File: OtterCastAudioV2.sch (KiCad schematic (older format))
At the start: 23 parts, among them J1 UART, J2 SD, U1 AllWinner-S3(FBGA-234), U2 AT24CS16-MAHM

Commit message: no drc error
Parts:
- R1, R10, R11, R12, R13, R2, R3, R4, R5, R6, R7, R8, R9: footprint otter:C_0402 -> otter:R_0402
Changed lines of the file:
@@
 F 0 "R7" V 11400 7750 50  0000 C CNN
 F 1 "47k" V 11400 8100 50  0000 C CNN
-F 2 "otter:C_0402" H 11450 7900 50  0001 C CNN
+F 2 "otter:R_0402" H 11450 7900 50  0001 C CNN
 F 3 "~" H 11450 7900 50  0001 C CNN
 	1    11450 7900
@@
 F 0 "R8" V 11400 7850 50  0000 C CNN
 F 1 "47k" V 11400 8200 50  0000 C CNN
-F 2 "otter:C_0402" H 11450 8000 50  0001 C CNN
+F 2 "otter:R_0402" H 11450 8000 50  0001 C CNN
 F 3 "~" H 11450 8000 50  0001 C CNN
 	1    11450 8000
@@
 F 0 "R9" V 11400 7950 50  0000 C CNN
 F 1 "47k" V 11400 8300 50  0000 C CNN
-F 2 "otter:C_0402" H 11450 8100 50  0001 C CNN
+F 2 "otter:R_0402" H 11450 8100 50  0001 C CNN
 F 3 "~" H 11450 8100 50  0001 C CNN
 	1    11450 8100
@@
 F 0 "R10" V 11400 8150 50  0000 C CNN
 F 1 "47k" V 11400 8500 50  0000 C CNN
-F 2 "otter:C_0402" H 11450 8300 50  0001 C CNN
+F 2 "otter:R_0402" H 11450 8300 50  0001 C CNN
 F 3 "~" H 11450 8300 50  0001 C CNN
 	1    11450 8300
@@
 F 0 "R11" V 11400 8350 50  0000 C CNN
 F 1 "47k" V 11400 8700 50  0000 C CNN
-F 2 "otter:C_0402" H 11450 8500 50  0001 C CNN
+F 2 "otter:R_0402" H 11450 8500 50  0001 C CNN
 F 3 "~" H 11450 8500 50  0001 C CNN
 	1    11450 8500
@@
 F 0 "R12" V 11400 8450 50  0000 C CNN
 F 1 "47k" V 11400 8800 50  0000 C CNN
-F 2 "otter:C_0402" H 11450 8600 50  0001 C CNN
+F 2 "otter:R_0402" H 11450 8600 50  0001 C CNN
 F 3 "~" H 11450 8600 50  0001 C CNN
 	1    11450 8600
@@
 F 0 "R13" V 11400 8550 50  0000 C CNN
 F 1 "47k" V 11400 8900 50  0000 C CNN
-F 2 "otter:C_0402" H 11450 8700 50  0001 C CNN
+F 2 "otter:R_0402" H 11450 8700 50  0001 C CNN
 F 3 "~" H 11450 8700 50  0001 C CNN
 	1    11450 8700
@@
 F 0 "R3" H 8041 10346 50  0000 R CNN
 F 1 "5k1" H 8041 10255 50  0000 R CNN
-F 2 "otter:C_0402" H 8100 10300 50  0001 C CNN
+F 2 "otter:R_0402" H 8100 10300 50  0001 C CNN
 F 3 "~" H 8100 10300 50  0001 C CNN
 	1    8100 10300
@@
 F 0 "R2" V 3950 6450 50  0000 C CNN
 F 1 "DNP" V 4000 6600 50  0000 C CNN
-F 2 "otter:C_0402" H 4000 6600 50  0001 C CNN
+F 2 "otter:R_0402" H 4000 6600 50  0001 C CNN
 F 3 "~" H 4000 6600 50  0001 C CNN
 	1    4000 6600
@@
 F 0 "R4" H 8391 10346 50  0000 R CNN
 F 1 "5k1" H 8391 10255 50  0000 R CNN
-F 2 "otter:C_0402" H 8450 10300 50  0001 C CNN
+F 2 "otter:R_0402" H 8450 10300 50  0001 C CNN
 F 3 "~" H 8450 10300 50  0001 C CNN
 	1    8450 10300
@@
 F 0 "R1" V 3646 2600 50  0000 C CNN
 F 1 "5k1" V 3555 2600 50  0000 C CNN
-F 2 "otter:C_0402" H 3450 2600 50  0001 C CNN
+F 2 "otter:R_0402" H 3450 2600 50  0001 C CNN
 F 3 "~" H 3450 2600 50  0001 C CNN
 	1    3450 2600
@@
 F 0 "R5" H 10609 10246 50  0000 L CNN
 F 1 "2.2k" H 10609 10155 50  0000 L CNN
-F 2 "otter:C_0402" H 10550 10200 50  0001 C CNN
+F 2 "otter:R_0402" H 10550 10200 50  0001 C CNN
 F 3 "~" H 10550 10200 50  0001 C CNN
 	1    10550 10200
@@
 F 0 "R6" H 10859 10246 50  0000 L CNN
 F 1 "2.2k" H 10859 10155 50  0000 L CNN
-F 2 "otter:C_0402" H 10800 10200 50  0001 C CNN
+F 2 "otter:R_0402" H 10800 10200 50  0001 C CNN
 F 3 "~" H 10800 10200 50  0001 C CNN
 	1    10800 10200

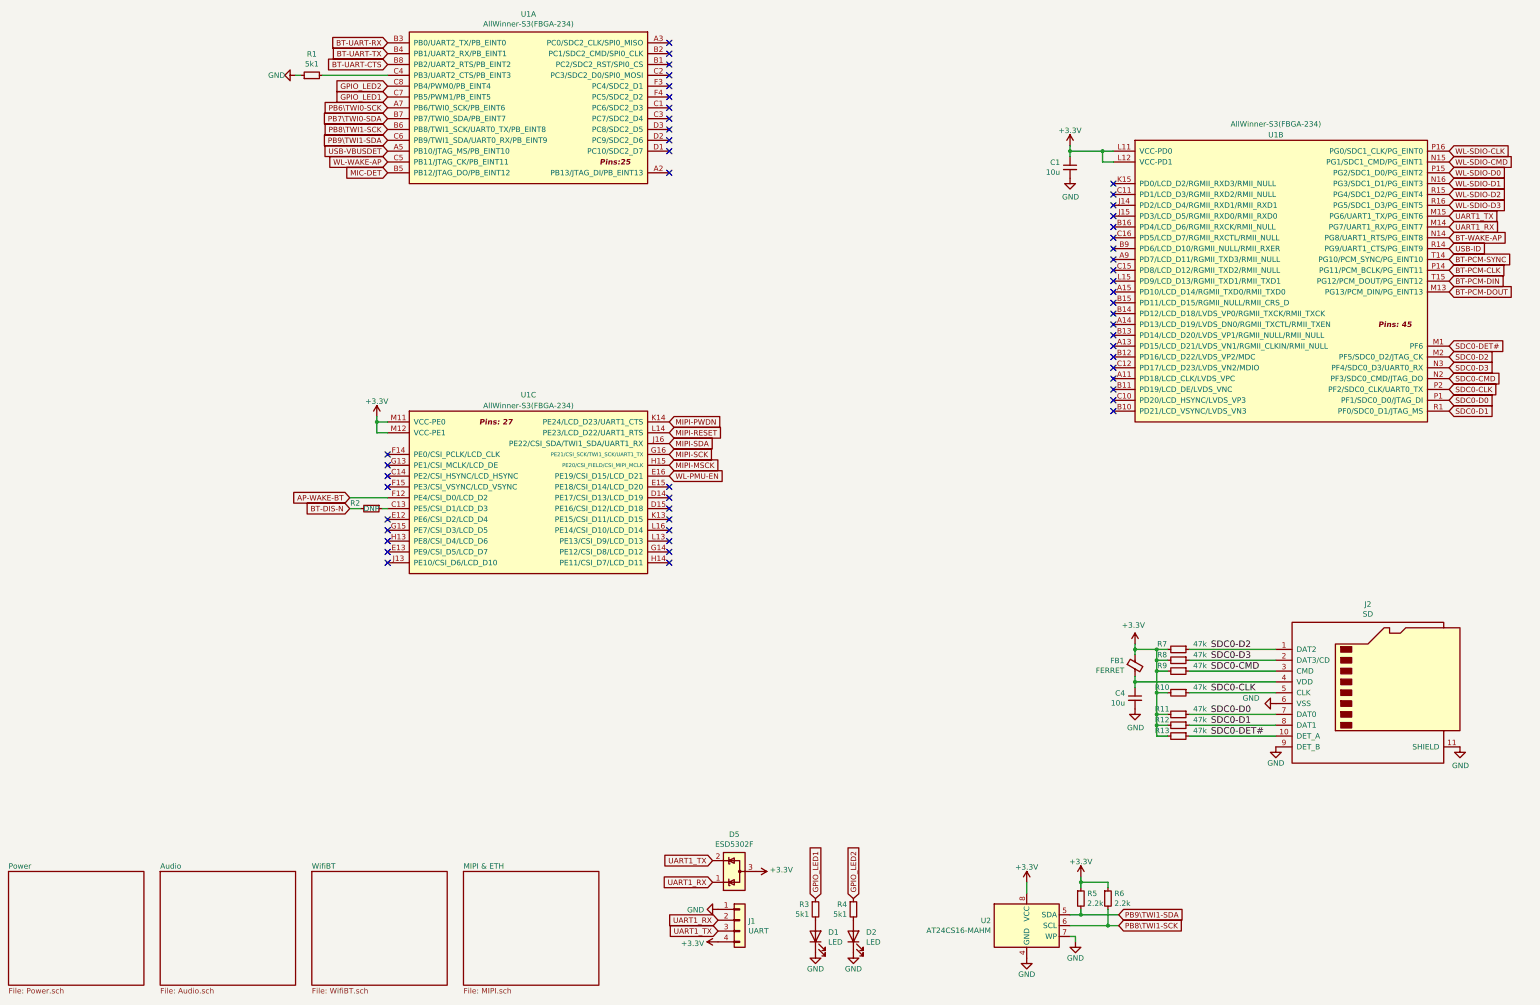
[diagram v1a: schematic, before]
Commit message: no drc error
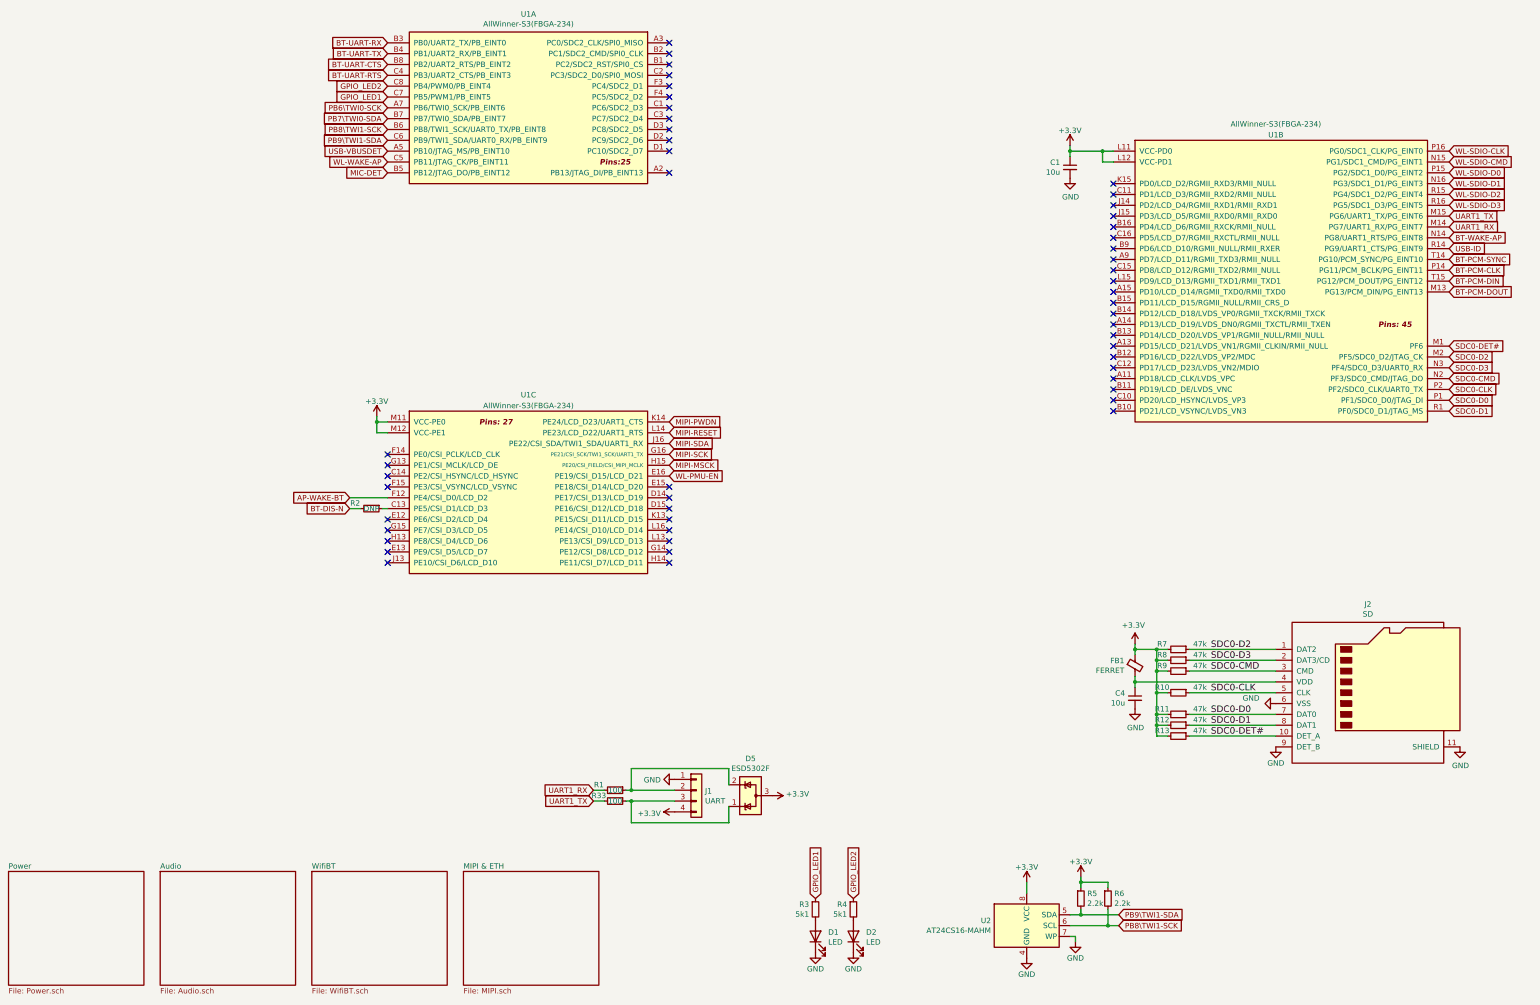
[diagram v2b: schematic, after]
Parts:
- added R33: 100, otter:R_0402, symbol Device:R_Small
- R1: value 5k1 -> 100
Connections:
- net GND: no longer R1.1
- net UART1_RX: now also R1.2; no longer D5.1 (K), J1.2 (Pin_2)
- net UART1_TX: now also R33.2; no longer D5.2 (K), J1.3 (Pin_3)
- net BT-UART-RTS: now reaches U1.C4 (PB3/UART2_CTS/PB_EINT3)
- net BT-UART-RTS: no longer R1.2
- new net: D5.1 (K), J1.3 (Pin_3), R33.1
- new net: D5.2 (K), J1.2 (Pin_2), R1.1
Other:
- moved on the sheet: D5, J1
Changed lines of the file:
@@
-$EndComp
-$Comp
-L S3-OLinuXino_Rev_A:GND #PWR03
-U 1 1 5D904B73
-P 3300 2600
-F 0 "#PWR03" H 3300 2350 50  0001 C CNN
-F 1 "GND" V 3300 2425 50  0000 C CNN
-F 2 "" H 3300 2600 60  0000 C CNN
-F 3 "" H 3300 2600 60  0000 C CNN
-	1    3300 2600
-	0    1    1    0
 $EndComp
 $Comp
@@
 L Connector_Generic:Conn_01x04 J1
 U 1 1 635CE136
-P 7400 10400
-F 0 "J1" H 7480 10392 50  0000 L CNN
-F 1 "UART" H 7480 10301 50  0000 L CNN
-F 2 "otter:PinHeader_1x04_P2.00mm_Vertical_nosilk_center" H 7400 10400 50  0001 C CNN
-F 3 "~" H 7400 10400 50  0001 C CNN
-	1    7400 10400
+P 7000 9200
+F 0 "J1" H 7080 9192 50  0000 L CNN
+F 1 "UART" H 7080 9101 50  0000 L CNN
+F 2 "otter:PinHeader_1x04_P2.00mm_Vertical_nosilk_center" H 7000 9200 50  0001 C CNN
+F 3 "~" H 7000 9200 50  0001 C CNN
+	1    7000 9200
 	1    0    0    -1
 $EndComp
@@
 L otter:GND #PWR0107
 U 1 1 635CE777
-P 7200 10300
-F 0 "#PWR0107" H 7200 10050 50  0001 C CNN
-F 1 "GND" V 7205 10172 50  0000 R CNN
-F 2 "" H 7200 10300 60  0000 C CNN
-F 3 "" H 7200 10300 60  0000 C CNN
-	1    7200 10300
-	0    1    1    0
-$EndComp
-Text GLabel 7200 10500 0    50   Input ~ 0
+P 6800 9100
+F 0 "#PWR0107" H 6800 8850 50  0001 C CNN
+F 1 "GND" V 6805 8972 50  0000 R CNN
+F 2 "" H 6800 9100 60  0000 C CNN
+F 3 "" H 6800 9100 60  0000 C CNN
+	1    6800 9100
+	0    1    1    0
+$EndComp
+Text GLabel 6050 9300 0    50   Input ~ 0
 UART1_TX
-Text GLabel 7200 10400 0    50   Input ~ 0
+Text GLabel 6050 9200 0    50   Input ~ 0
 UART1_RX
 $Comp
 L S3-OLinuXino_Rev_A:+3.3V #PWR0108
 U 1 1 63623CC5
-P 7200 10600
-F 0 "#PWR0108" H 7200 10450 50  0001 C CNN
-F 1 "+3.3V" V 7215 10728 50  0000 L CNN
-F 2 "" H 7200 10600 60  0000 C CNN
-F 3 "" H 7200 10600 60  0000 C CNN
-	1    7200 10600
+P 6800 9400
+F 0 "#PWR0108" H 6800 9250 50  0001 C CNN
+F 1 "+3.3V" V 6815 9528 50  0000 L CNN
+F 2 "" H 6800 9400 60  0000 C CNN
+F 3 "" H 6800 9400 60  0000 C CNN
+	1    6800 9400
 	0    -1   1    0
 $EndComp
@@
 Text GLabel 4150 2500 0    50   Input ~ 0
 BT-UART-CTS
-$Comp
-L Device:R_Small R1
-U 1 1 67C10E27
-P 3450 2600
-F 0 "R1" V 3646 2600 50  0000 C CNN
-F 1 "5k1" V 3555 2600 50  0000 C CNN
-F 2 "otter:R_0402" H 3450 2600 50  0001 C CNN
-F 3 "~" H 3450 2600 50  0001 C CNN
-	1    3450 2600
-	0    -1   -1   0
-$EndComp
-Wire Wire Line
-	3300 2600 3350 2600
-Wire Wire Line
-	3550 2600 4150 2600
 Text GLabel 4150 2900 0    50   Input ~ 0
 PB6\TWI0-SCK
@@
 L Power_Protection:SP0502BAHT D5
 U 1 1 5FCE3FA8
-P 7350 9950
-F 0 "D5" V 7692 9950 50  0000 C CNN
-F 1 "ESD5302F" V 7601 9950 50  0000 C CNN
-F 2 "Package_TO_SOT_SMD:SOT-23" H 7575 9900 50  0001 L CNN
-F 3 "http://www.littelfuse.com/~/media/files/littelfuse/technical%20resources/documents/data%20sheets/sp05xxba.pdf" H 7475 10075 50  0001 C CNN
-F 4 "C239643" V 7350 9950 50  0001 C CNN "LCSC"
-	1    7350 9950
+P 7500 9250
+F 0 "D5" V 7842 9250 50  0000 C CNN
+F 1 "ESD5302F" V 7751 9250 50  0000 C CNN
+F 2 "Package_TO_SOT_SMD:SOT-23" H 7725 9200 50  0001 L CNN
+F 3 "http://www.littelfuse.com/~/media/files/littelfuse/technical%20resources/documents/data%20sheets/sp05xxba.pdf" H 7625 9375 50  0001 C CNN
+F 4 "C239643" V 7500 9250 50  0001 C CNN "LCSC"
+	1    7500 9250
 	0    -1   -1   0
 $EndComp
-Text GLabel 7150 9850 0    50   Input ~ 0
-UART1_TX
-Text GLabel 7150 10050 0    50   Input ~ 0
-UART1_RX
 $Comp
 L S3-OLinuXino_Rev_A:+3.3V #PWR0154
 U 1 1 5FCE77D5
-P 7550 9950
-F 0 "#PWR0154" H 7550 9800 50  0001 C CNN
-F 1 "+3.3V" V 7565 10078 50  0000 L CNN
-F 2 "" H 7550 9950 60  0000 C CNN
-F 3 "" H 7550 9950 60  0000 C CNN
-	1    7550 9950
+P 7700 9250
+F 0 "#PWR0154" H 7700 9100 50  0001 C CNN
+F 1 "+3.3V" V 7715 9378 50  0000 L CNN
+F 2 "" H 7700 9250 60  0000 C CNN
+F 3 "" H 7700 9250 60  0000 C CNN
+	1    7700 9250
 	0    1    -1   0
 $EndComp
 Wire Wire Line
 	10050 10050 10050 10150
+Text GLabel 4150 2600 0    50   Input ~ 0
+BT-UART-RTS
+$Comp
+L Device:R_Small R1
+U 1 1 5FE69B36
+P 6250 9200
+F 0 "R1" V 6200 9050 50  0000 C CNN
+F 1 "100" V 6250 9200 50  0000 C CNN
+F 2 "otter:R_0402" H 6250 9200 50  0001 C CNN
+F 3 "~" H 6250 9200 50  0001 C CNN
+	1    6250 9200
+	0    1    1    0
+$EndComp
+$Comp
+L Device:R_Small R33
+U 1 1 5FE69B3C
+P 6250 9300
+F 0 "R33" V 6200 9150 50  0000 C CNN
+F 1 "100" V 6250 9300 50  0000 C CNN
+F 2 "otter:R_0402" H 6250 9300 50  0001 C CNN
+F 3 "~" H 6250 9300 50  0001 C CNN
+	1    6250 9300
+	0    1    1    0
+$EndComp
+Wire Wire Line
+	6050 9200 6150 9200
+Wire Wire Line
+	6050 9300 6150 9300
+Wire Wire Line
+	6350 9200 6400 9200
+Wire Wire Line
+	6350 9300 6400 9300
+Wire Wire Line
+	6400 9300 6400 9500
+Wire Wire Line
+	6400 9500 7300 9500
+Wire Wire Line
+	7300 9500 7300 9350
+Connection ~ 6400 9300
+Wire Wire Line
+	6400 9300 6800 9300
+Wire Wire Line
+	6400 9200 6400 9000
+Wire Wire Line
+	6400 9000 7300 9000
+Wire Wire Line
+	7300 9000 7300 9150
+Connection ~ 6400 9200
+Wire Wire Line
+	6400 9200 6800 9200
 $EndSCHEMATC
